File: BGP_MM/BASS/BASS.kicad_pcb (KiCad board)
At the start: 2 copper layers, 24 x 21 mm, 8 parts, among them J1 Conn_01x02_Male, J2 Conn_01x02_Male, J3 Conn_01x04_Male, J4 Conn_01x04_Male, P2 Conn_01x02, P3 Conn_01x02, P4 Conn_01x03

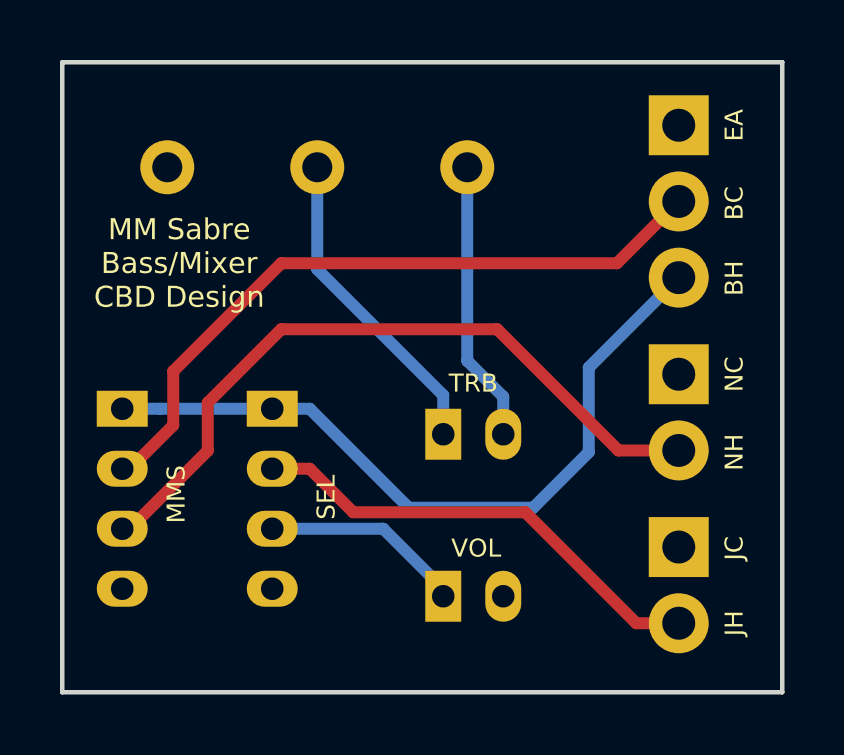
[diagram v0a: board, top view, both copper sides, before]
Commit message: MM Gerbers, BASS pot fixup
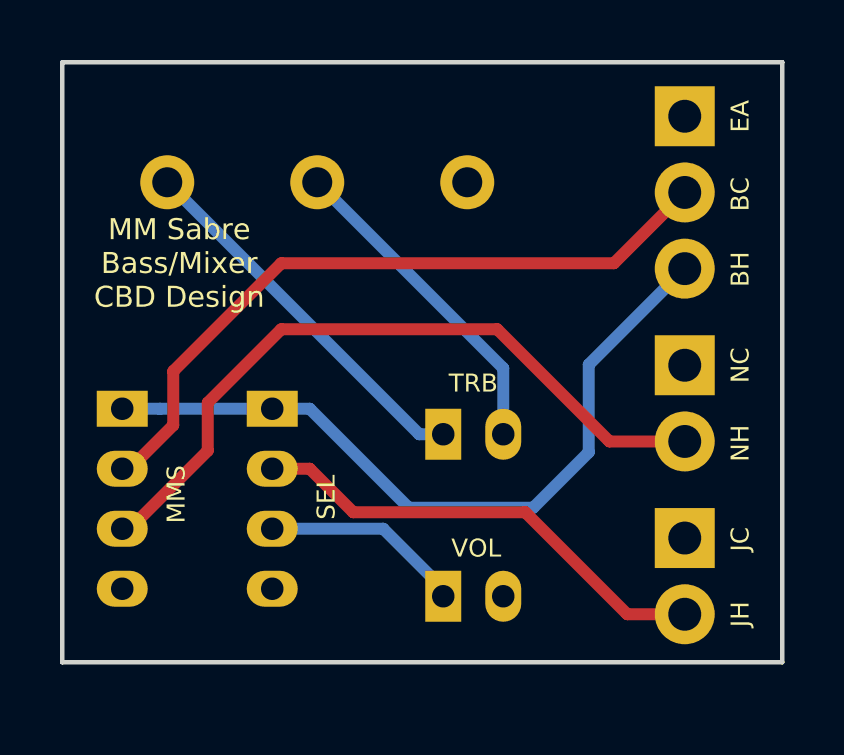
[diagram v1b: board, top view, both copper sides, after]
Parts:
- moved RV1 0.50 mm to (137.5, 85.0)
- moved P3 0.36 mm to (149.8, 91.1)
- moved P2 0.36 mm to (149.8, 96.9)
- moved P4 0.36 mm to (149.8, 82.8)
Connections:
- RV1 pad 1: Net-(RV1-Pad1) -> Net-(J1-Pad1)
- RV1 pad 2: Net-(J1-Pad1) -> Net-(J1-Pad2)
- RV1 pad 3: Net-(J1-Pad2) -> Net-(RV1-Pad3)
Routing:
- net Net-(J1-Pad1): track 10.6 -> 12.7 mm
- net Net-(J1-Pad2): track 9.40 -> 11.0 mm
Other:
- board size 24 x 21 mm -> 24 x 20 mm
